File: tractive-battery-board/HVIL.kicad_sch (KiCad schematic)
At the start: 13 parts, among them J13 TS, J14 HVIL+/HVIL-, U17 MCP6004

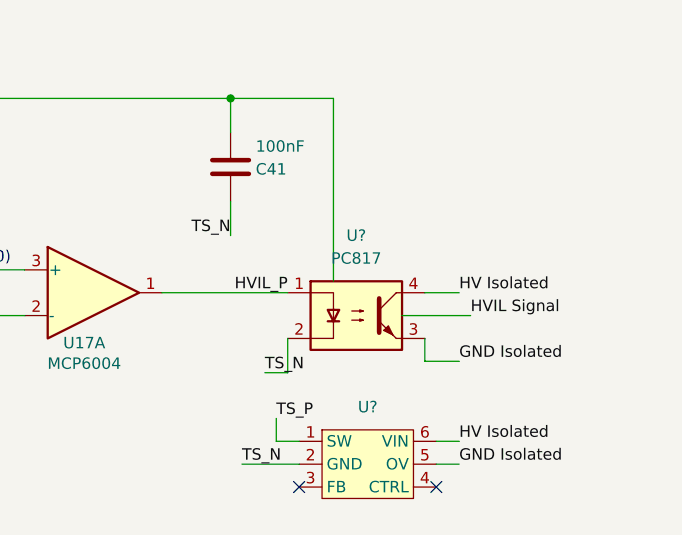
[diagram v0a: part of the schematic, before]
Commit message: Fixed MCU PINs
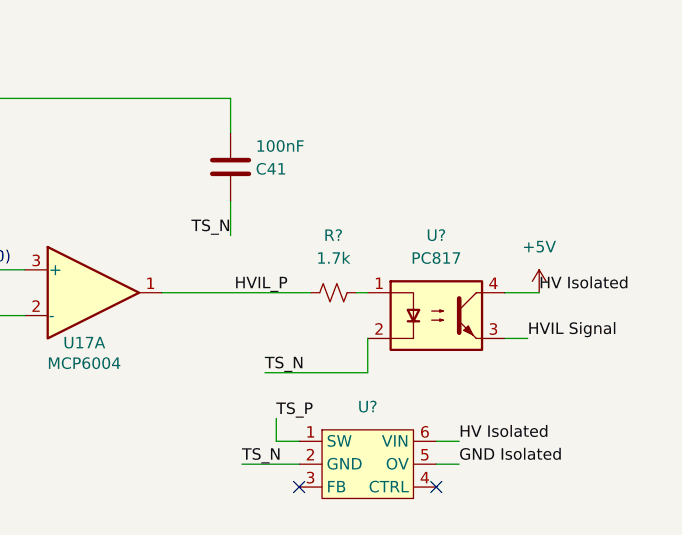
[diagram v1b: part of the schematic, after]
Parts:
- added R?: 1.7k, symbol Device:R_Small_US
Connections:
- net GND Isolated: no longer U?.3
- net HVIL Signal: now also U?.3
- net HVIL_P: now also R?.1; no longer U?.1
- net HV Isolated renamed +5V
- new net: R?.2, U?.1
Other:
- moved on the sheet: U?

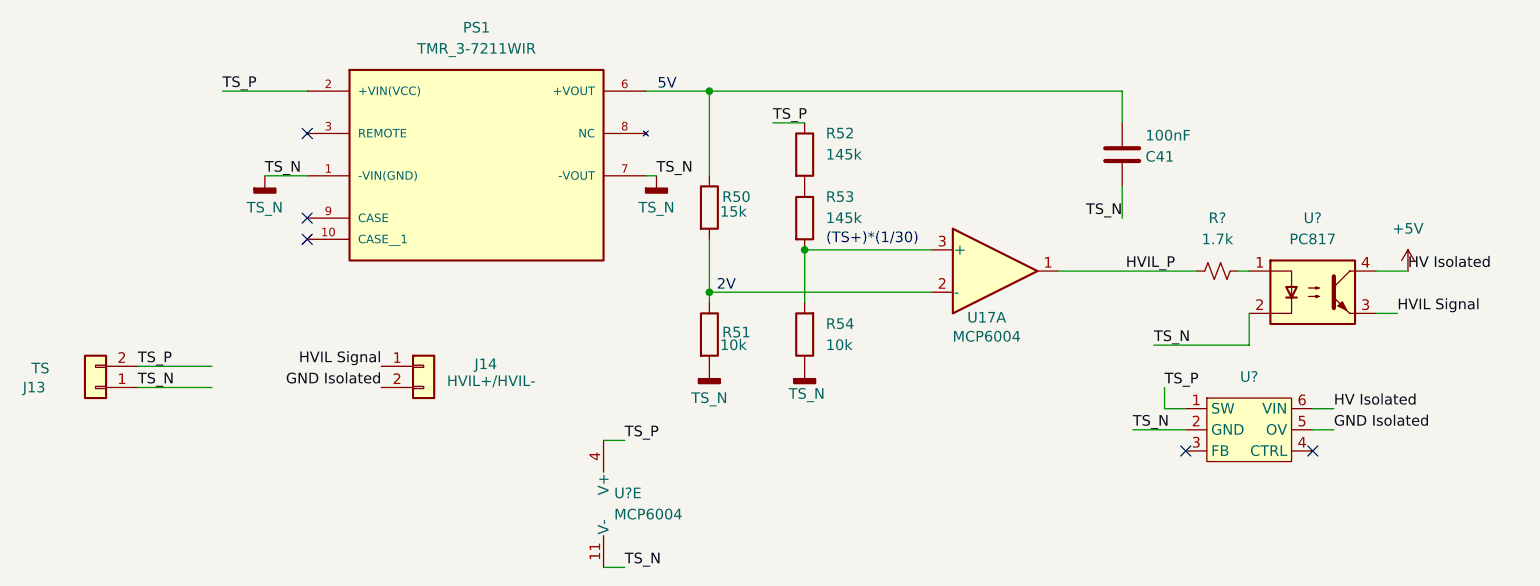
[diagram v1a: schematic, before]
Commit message: Removed Isolation from HVIL
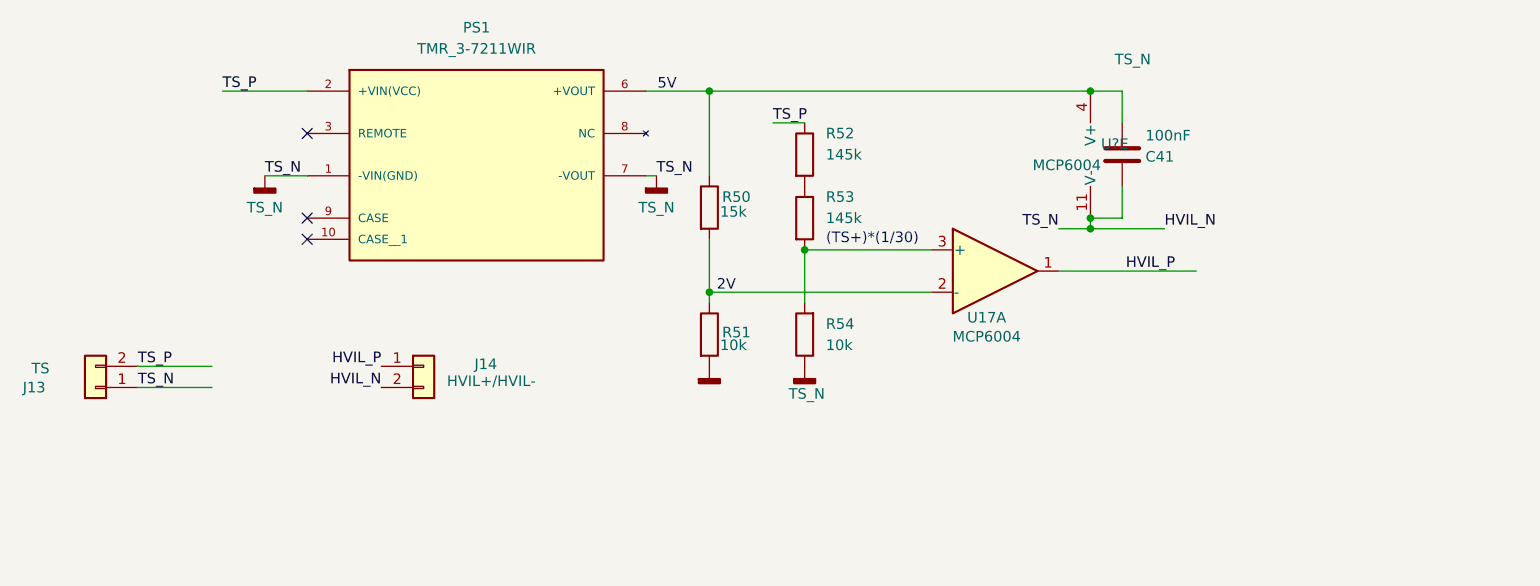
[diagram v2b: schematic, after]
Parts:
- removed R?: 1.7k, symbol Device:R_Small_US
- removed U?: (no value), Package_TO_SOT_SMD:SOT-23-6_Handsoldering, symbol formula_slug_symbol_library:AP3032KTR-G1
- removed U?: PC817, Package_DIP:DIP-4_W7.62mm, symbol Isolator:PC817
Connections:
- net GND Isolated is gone; now on net TS_N: J14.2 (Pin_2)
- net HVIL Signal is gone; now on net HVIL_P: J14.1 (Pin_1)
- net TS_P: no longer U?.4 (V+)
- net at C41.2, PS1.6 (+VOUT), R50.1: now also U?.4 (V+)
- no-connect marks 5 -> 3
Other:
- moved on the sheet: U?E
